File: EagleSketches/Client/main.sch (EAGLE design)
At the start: 15 parts

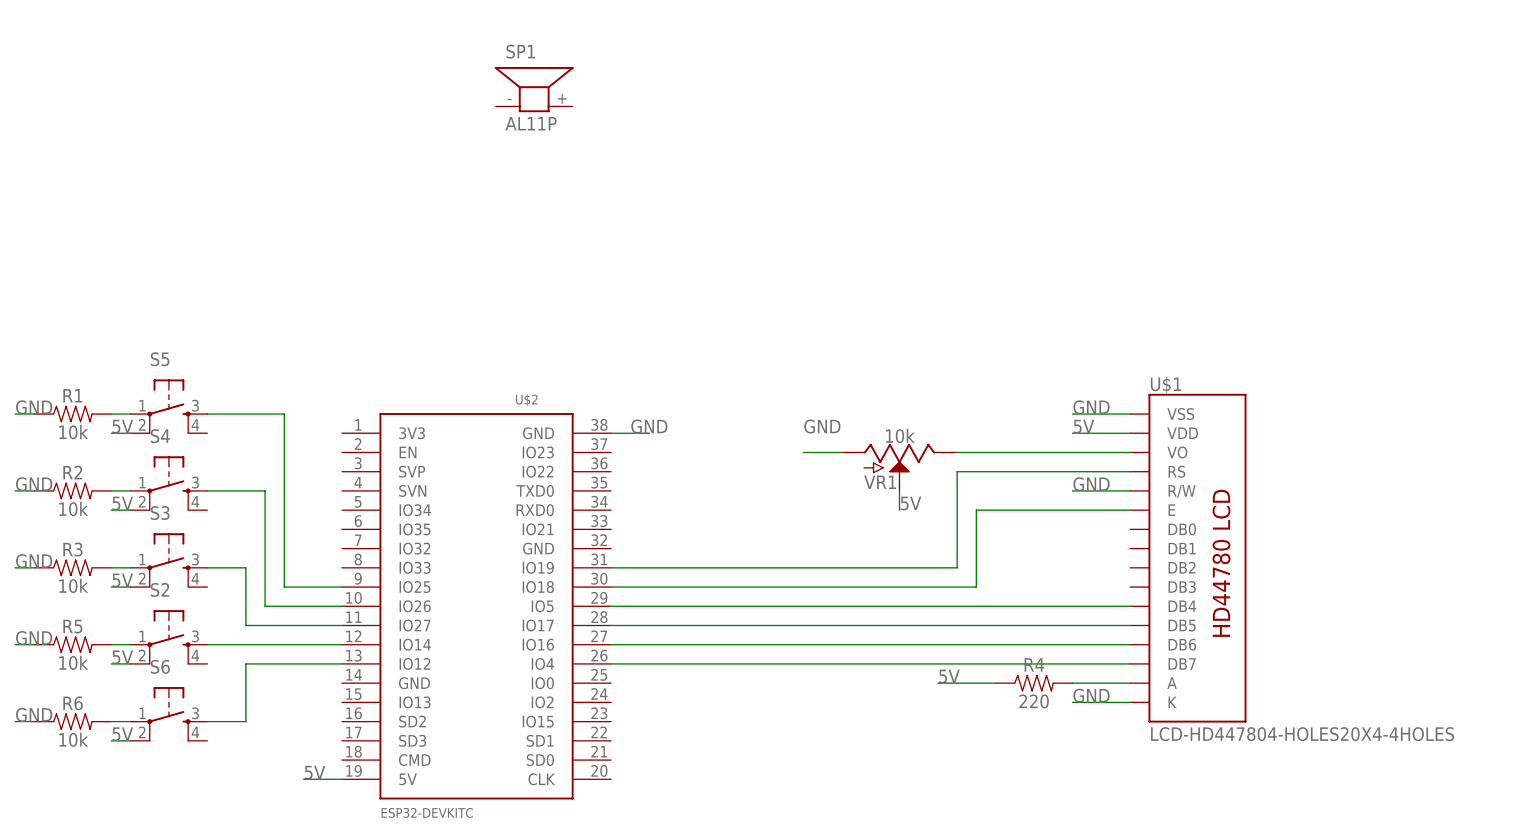
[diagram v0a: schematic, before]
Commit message: Nye UUID's og eagle ændringer
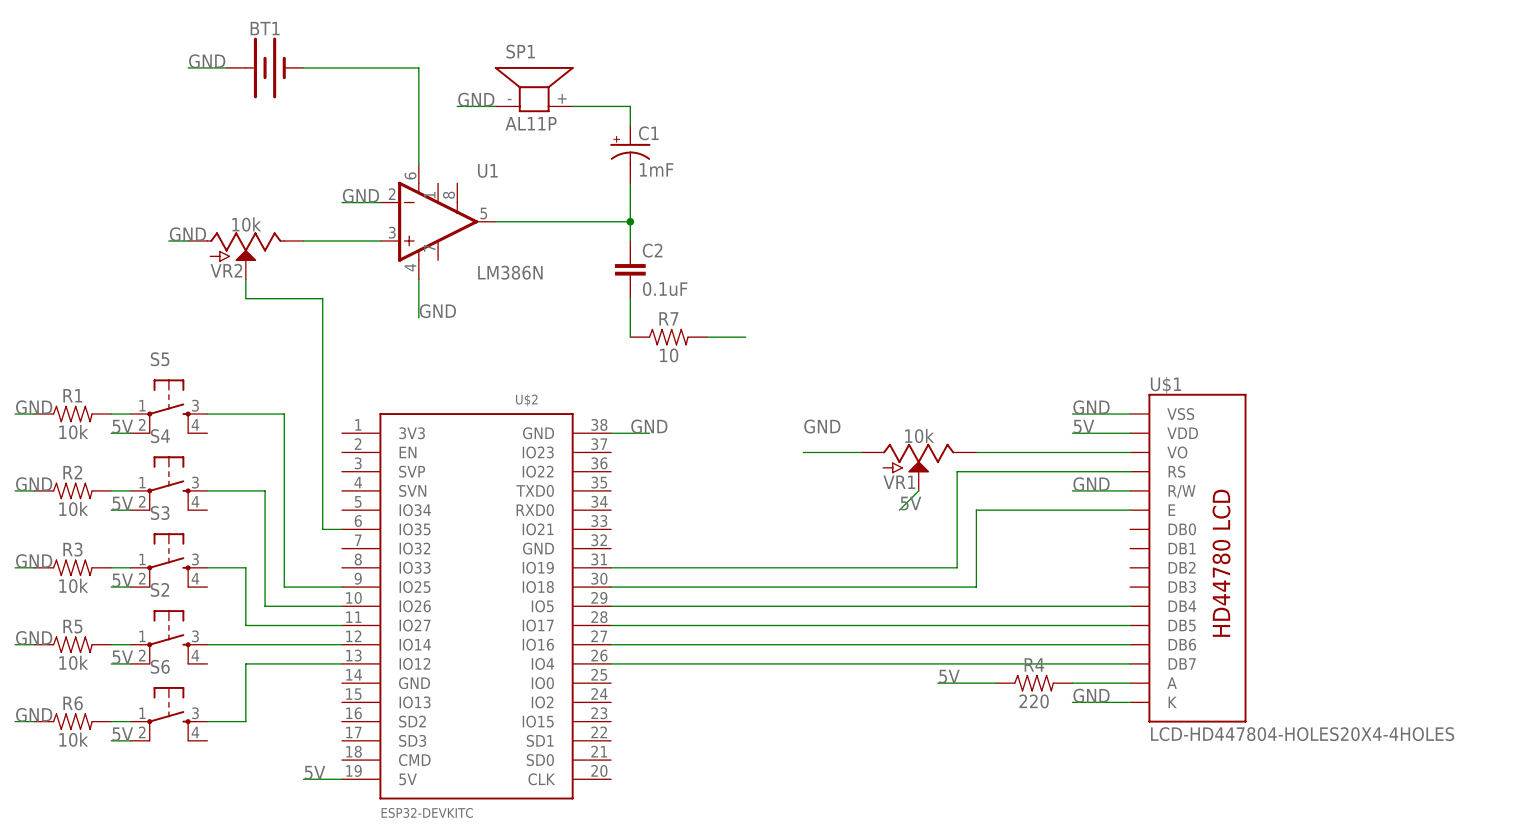
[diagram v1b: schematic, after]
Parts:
- added BT1: (no value), SparkFun-Batteries:BATTERY-9V
- added C1: 1mF, SparkFun-Capacitors:1000UF-RADIAL-5MM-25V-20%
- added C2: 0.1uF, SparkFun-Capacitors:0.1UF-KIT-EZ-50V-20%
- added R7: 10, SparkFun-Resistors:10OHM-HORIZ-1/4W-1%
- added U1: LM386N, SparkFun-IC-Amplifiers:LM386
- added VR2: 10k, SparkFun-Resistors:POTENTIOMETER_SLIDE-60MM-1/2W-20%
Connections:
- new net N$11: C1.+, SP1.2
- new net N$13: C1.-, C2.1, U1.OUT
- new net N$19: C2.2, R7.1
- new net N$20: R7.2
- new net N$21: U$2.IO35, VR2.S
- new net N$22: BT1.-, U1.V+
- new net N$23: U1.+IN, VR2.E
- net GND: now also BT1.+, SP1.1, U1.-IN, U1.V-, VR2.A
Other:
- moved on the sheet: VR1
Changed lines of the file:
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@@
 <layer number="56" name="wert" color="7" fill="1" visible="no" active="no"/>
 <layer number="57" name="tCAD" color="7" fill="1" visible="no" active="no"/>
+<layer number="58" name="bCopper" color="7" fill="1" visible="no" active="no"/>
 <layer number="59" name="tCarbon" color="7" fill="1" visible="no" active="no"/>
 <layer number="60" name="bCarbon" color="7" fill="1" visible="no" active="no"/>
@@
 <layer number="250" name="Descript" color="3" fill="1" visible="no" active="no"/>
 <layer number="251" name="SMDround" color="12" fill="11" visible="no" active="no"/>
+<layer number="253" name="Extra" color="7" fill="1" visible="no" active="no"/>
 <layer number="254" name="cooling" color="7" fill="1" visible="no" active="no"/>
 <layer number="255" name="routoute" color="7" fill="1" visible="no" active="no"/>
@@
 <part name="R6" library="SparkFun-Resistors" deviceset="10KOHM" device="-HORIZ-1/4W-1%" value="10k"/>
 <part name="SP1" library="buzzer" library_urn="urn:adsk.eagle:library:113" deviceset="AL11P" device="" package3d_urn="urn:adsk.eagle:package:5308/1"/>
+<part name="R7" library="SparkFun-Resistors" deviceset="10OHM" device="-HORIZ-1/4W-1%" value="10"/>
+<part name="C1" library="SparkFun-Capacitors" deviceset="1000UF" device="-RADIAL-5MM-25V-20%" value="1mF"/>
+<part name="C2" library="SparkFun-Capacitors" deviceset="0.1UF" device="-KIT-EZ-50V-20%" value="0.1uF"/>
+<part name="U1" library="SparkFun-IC-Amplifiers" deviceset="LM386" device="" value="LM386N"/>
+<part name="VR2" library="SparkFun-Resistors" deviceset="POTENTIOMETER_SLIDE" device="-60MM-1/2W-20%" value="10k"/>
+<part name="BT1" library="SparkFun-Batteries" deviceset="BATTERY" device="-9V"/>
 </parts>
 <sheets>
@@
 </plain>
 <instances>
-<instance part="VR1" gate="G$1" x="40.64" y="83.82" smashed="yes" rot="R270">
-<attribute name="NAME" x="40.386" y="80.772" size="1.778" layer="95" font="vector" rot="R180"/>
-<attribute name="VALUE" x="40.64" y="85.09" size="1.778" layer="95" font="vector" align="bottom-center"/>
+<instance part="VR1" gate="G$1" x="43.18" y="83.82" smashed="yes" rot="R270">
+<attribute name="NAME" x="42.926" y="80.772" size="1.778" layer="95" font="vector" rot="R180"/>
+<attribute name="VALUE" x="43.18" y="85.09" size="1.778" layer="95" font="vector" align="bottom-center"/>
 </instance>
 <instance part="U$1" gate="G$1" x="81.28" y="68.58" smashed="yes">
@@
 <attribute name="NAME" x="-11.43" y="135.89" size="1.778" layer="95"/>
 <attribute name="VALUE" x="-11.43" y="126.365" size="1.778" layer="96"/>
+</instance>
+<instance part="R7" gate="G$1" x="10.16" y="99.06" smashed="yes">
+<attribute name="NAME" x="10.16" y="100.584" size="1.778" layer="95" font="vector" align="bottom-center"/>
+<attribute name="VALUE" x="10.16" y="97.536" size="1.778" layer="96" font="vector" align="top-center"/>
+</instance>
+<instance part="C1" gate="G$1" x="5.08" y="124.46" smashed="yes">
+<attribute name="NAME" x="6.096" y="125.095" size="1.778" layer="95" font="vector"/>
+<attribute name="VALUE" x="6.096" y="120.269" size="1.778" layer="96" font="vector"/>
+</instance>
+<instance part="C2" gate="G$1" x="5.08" y="106.68" smashed="yes">
+<attribute name="NAME" x="6.604" y="109.601" size="1.778" layer="95" font="vector"/>
+<attribute name="VALUE" x="6.604" y="104.521" size="1.778" layer="96" font="vector"/>
+</instance>
+<instance part="U1" gate="G1" x="-22.86" y="114.3" smashed="yes">
+<attribute name="NAME" x="-15.24" y="120.142" size="1.778" layer="95" font="vector"/>
+<attribute name="VALUE" x="-15.24" y="106.68" size="1.778" layer="95" font="vector"/>
+</instance>
+<instance part="VR2" gate="G$1" x="-45.72" y="111.76" smashed="yes" rot="R270">
+<attribute name="NAME" x="-45.974" y="108.712" size="1.778" layer="95" font="vector" rot="R180"/>
+<attribute name="VALUE" x="-45.72" y="113.03" size="1.778" layer="95" font="vector" align="bottom-center"/>
+</instance>
+<instance part="BT1" gate="G$1" x="-43.18" y="134.62" smashed="yes">
+<attribute name="NAME" x="-43.18" y="138.938" size="1.778" layer="95" font="vector" align="bottom-center"/>
+<attribute name="VALUE" x="-43.18" y="130.302" size="1.778" layer="96" font="vector" align="top-center"/>
 </instance>
 </instances>
@@
 <segment>
 <pinref part="VR1" gate="G$1" pin="A"/>
-<wire x1="33.02" y1="83.82" x2="27.94" y2="83.82" width="0.1524" layer="91"/>
+<wire x1="35.56" y1="83.82" x2="27.94" y2="83.82" width="0.1524" layer="91"/>
 <label x="27.94" y="86.36" size="1.778" layer="95"/>
 </segment>
@@
 <label x="-76.2" y="78.74" size="1.778" layer="95"/>
 </segment>
+<segment>
+<pinref part="SP1" gate="G$1" pin="1"/>
+<wire x1="-12.7" y1="129.54" x2="-17.78" y2="129.54" width="0.1524" layer="91"/>
+<label x="-17.78" y="129.54" size="1.778" layer="95"/>
+</segment>
+<segment>
+<pinref part="VR2" gate="G$1" pin="A"/>
+<wire x1="-53.34" y1="111.76" x2="-55.88" y2="111.76" width="0.1524" layer="91"/>
+<label x="-55.88" y="111.76" size="1.778" layer="95"/>
+</segment>
+<segment>
+<pinref part="U1" gate="G1" pin="V-"/>
+<wire x1="-22.86" y1="106.68" x2="-22.86" y2="101.6" width="0.1524" layer="91"/>
+<label x="-22.86" y="101.6" size="1.778" layer="95"/>
+</segment>
+<segment>
+<pinref part="U1" gate="G1" pin="-IN"/>
+<wire x1="-27.94" y1="116.84" x2="-33.02" y2="116.84" width="0.1524" layer="91"/>
+<label x="-33.02" y="116.84" size="1.778" layer="95"/>
+</segment>
+<segment>
+<pinref part="BT1" gate="G$1" pin="+"/>
+<wire x1="-48.26" y1="134.62" x2="-53.34" y2="134.62" width="0.1524" layer="91"/>
+<label x="-53.34" y="134.62" size="1.778" layer="95"/>
+</segment>
 </net>
 <net name="5V" class="0">
@@
 <segment>
 <pinref part="VR1" gate="G$1" pin="S"/>
-<wire x1="40.64" y1="78.74" x2="40.64" y2="76.2" width="0.1524" layer="91"/>
+<wire x1="43.18" y1="78.74" x2="40.64" y2="76.2" width="0.1524" layer="91"/>
 <label x="40.64" y="76.2" size="1.778" layer="95"/>
 </segment>
@@
 <pinref part="U$1" gate="G$1" pin="VO"/>
 <pinref part="VR1" gate="G$1" pin="E"/>
-<wire x1="71.12" y1="83.82" x2="48.26" y2="83.82" width="0.1524" layer="91"/>
+<wire x1="71.12" y1="83.82" x2="50.8" y2="83.82" width="0.1524" layer="91"/>
 </segment>
 </net>
@@
 </segment>
 </net>
+<net name="N$11" class="0">
+<segment>
+<pinref part="SP1" gate="G$1" pin="2"/>
+<wire x1="-2.54" y1="129.54" x2="5.08" y2="129.54" width="0.1524" layer="91"/>
+<pinref part="C1" gate="G$1" pin="+"/>
+<wire x1="5.08" y1="129.54" x2="5.08" y2="127" width="0.1524" layer="91"/>
+</segment>
+</net>
+<net name="N$13" class="0">
+<segment>
+<pinref part="U1" gate="G1" pin="OUT"/>
+<pinref part="C1" gate="G$1" pin="-"/>
+<wire x1="-12.7" y1="114.3" x2="5.08" y2="114.3" width="0.1524" layer="91"/>
+<wire x1="5.08" y1="114.3" x2="5.08" y2="119.38" width="0.1524" layer="91"/>
+<pinref part="C2" gate="G$1" pin="1"/>
+<wire x1="5.08" y1="114.3" x2="5.08" y2="111.76" width="0.1524" layer="91"/>
+<junction x="5.08" y="114.3"/>
+</segment>
+</net>
+<net name="N$19" class="0">
+<segment>
+<pinref part="C2" gate="G$1" pin="2"/>
+<pinref part="R7" gate="G$1" pin="1"/>
+<wire x1="5.08" y1="104.14" x2="5.08" y2="99.06" width="0.1524" layer="91"/>
+</segment>
+</net>
+<net name="N$20" class="0">
+<segment>
+<pinref part="R7" gate="G$1" pin="2"/>
+<wire x1="15.24" y1="99.06" x2="20.32" y2="99.06" width="0.1524" layer="91"/>
+</segment>
+</net>
+<net name="N$23" class="0">
+<segment>
+<pinref part="VR2" gate="G$1" pin="E"/>
+<pinref part="U1" gate="G1" pin="+IN"/>
+<wire x1="-38.1" y1="111.76" x2="-27.94" y2="111.76" width="0.1524" layer="91"/>
+</segment>
+</net>
+<net name="N$21" class="0">
+<segment>
+<pinref part="U$2" gate="G$1" pin="IO35"/>
+<wire x1="-33.02" y1="73.66" x2="-35.56" y2="73.66" width="0.1524" layer="91"/>
+<wire x1="-35.56" y1="73.66" x2="-35.56" y2="104.14" width="0.1524" layer="91"/>
+<pinref part="VR2" gate="G$1" pin="S"/>
+<wire x1="-35.56" y1="104.14" x2="-45.72" y2="104.14" width="0.1524" layer="91"/>
+<wire x1="-45.72" y1="104.14" x2="-45.72" y2="106.68" width="0.1524" layer="91"/>
+</segment>
+</net>
+<net name="N$22" class="0">
+<segment>
+<pinref part="BT1" gate="G$1" pin="-"/>
+<wire x1="-38.1" y1="134.62" x2="-22.86" y2="134.62" width="0.1524" layer="91"/>
+<pinref part="U1" gate="G1" pin="V+"/>
+<wire x1="-22.86" y1="134.62" x2="-22.86" y2="121.92" width="0.1524" layer="91"/>
+</segment>
+</net>
